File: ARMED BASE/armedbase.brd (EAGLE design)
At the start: 160 x 100 mm, 21 parts, among them K1 CQ1-12V, X1 RJ45-6L2-B, X2 RJ45-6L2-B

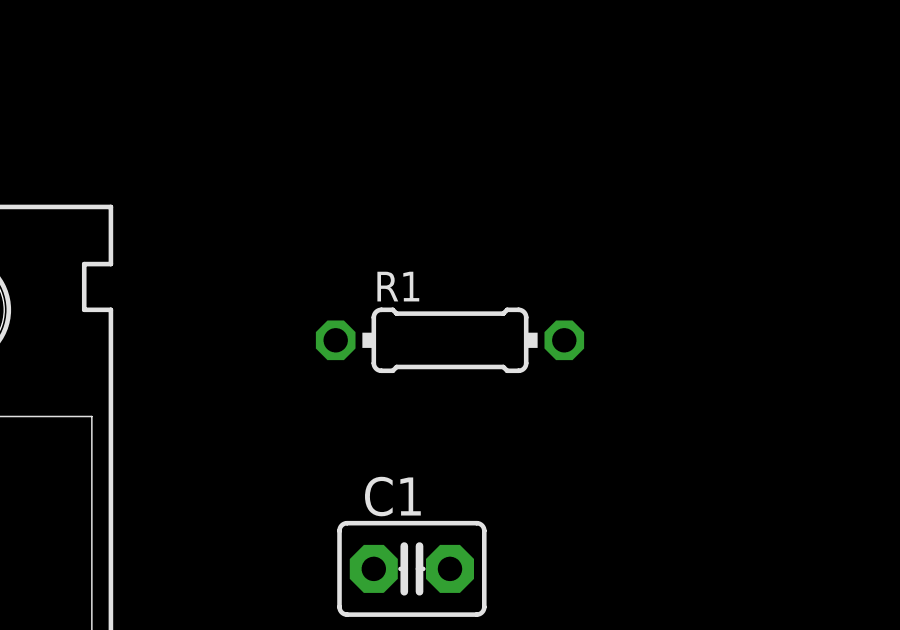
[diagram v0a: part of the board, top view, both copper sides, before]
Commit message: smd
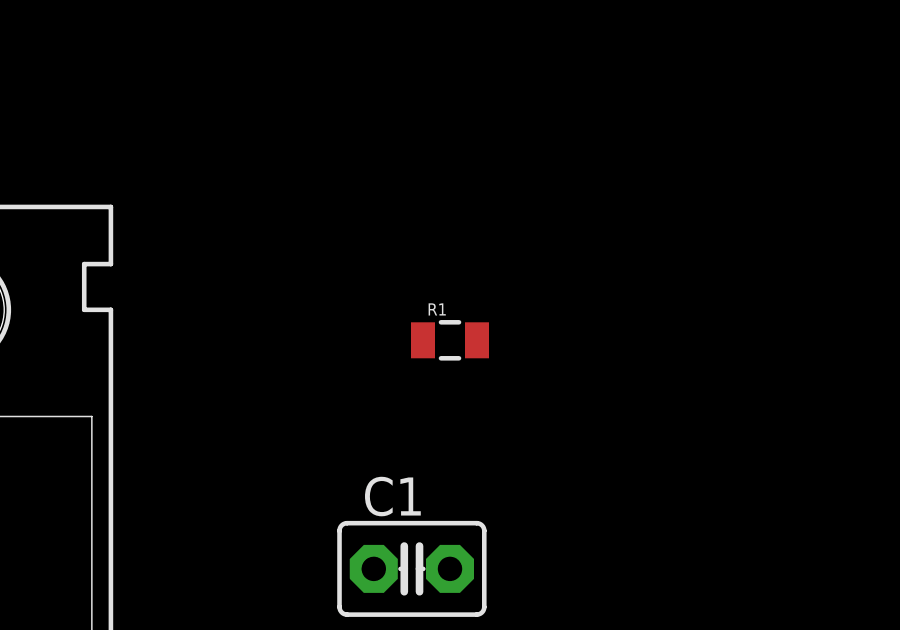
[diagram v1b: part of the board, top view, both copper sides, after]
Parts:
- R1: device eagle-ltspice:0204/7 -> SparkFun-Passives:0805
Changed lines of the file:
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@@
 <element name="IC1" library="SparkFun-PowerIC" package="78XXL" value="" x="26.67" y="11.43"/>
 <element name="Q1" library="SparkFun-DiscreteSemi" package="TO-92-AMMO" value="" x="133.35" y="27.94"/>
-<element name="R1" library="eagle-ltspice" package="0204/7" value="" x="43.18" y="21.59">
-<attribute name="SPICEMODEL" value="NONE" x="90.17" y="-39.37" size="1.778" layer="27" display="off"/>
-<attribute name="SPICEPREFIX" value="R" x="90.17" y="-39.37" size="1.778" layer="27" display="off"/>
-</element>
+<element name="R1" library="SparkFun-Passives" package="0805" value="" x="43.18" y="21.59"/>
 <element name="C1" library="capacitor-wima" package="C2.5-3" value="" x="41.91" y="13.97"/>
 <element name="LED1" library="led" package="LED5MM" value="" x="6.35" y="22.86"/>
